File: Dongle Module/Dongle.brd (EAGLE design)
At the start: 45 x 28 mm, 31 parts, among them Q2 2.5A/30V, U1 RFM69HCW, U10 74AHC1G125, U8 ATSAMD21G-A, U9 3.3V, Y1 32.768kHz

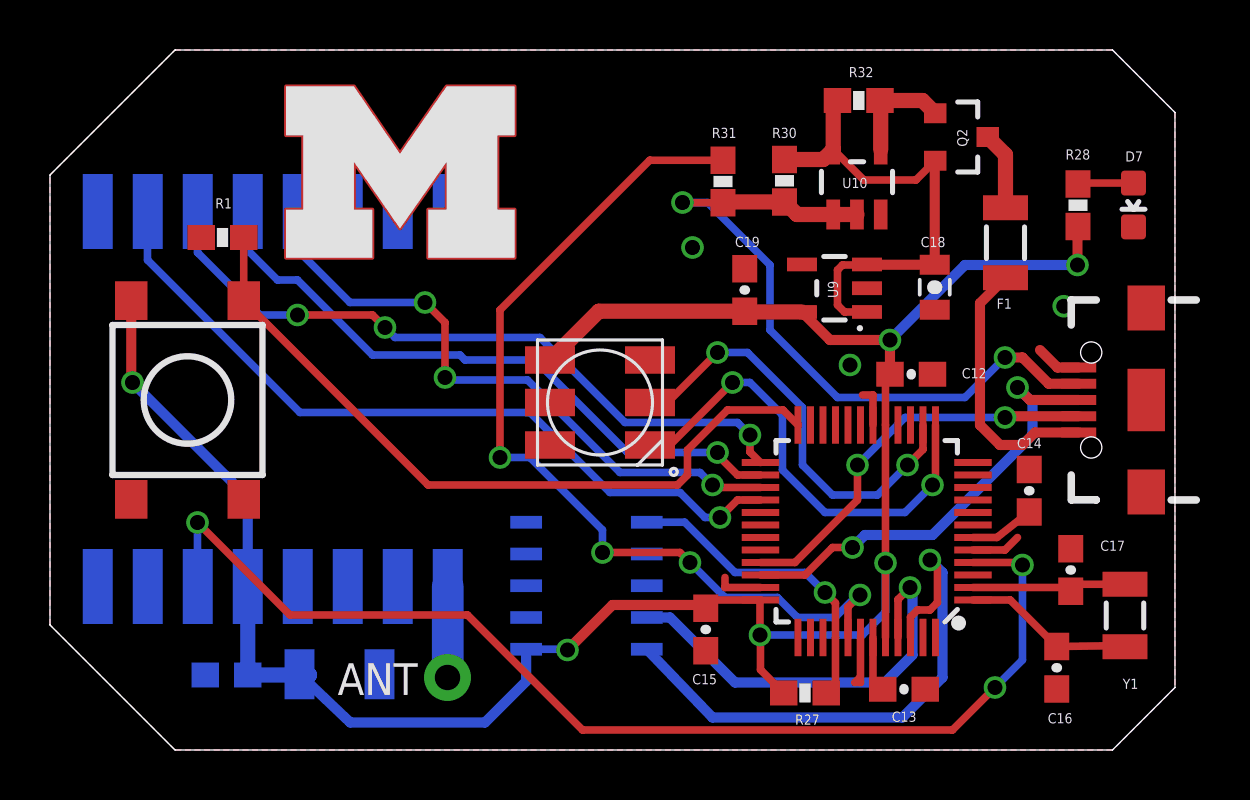
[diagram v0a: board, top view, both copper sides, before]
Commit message: ACTUALLY finalized all of the PCBs and created .zip's containing the gerber files of each
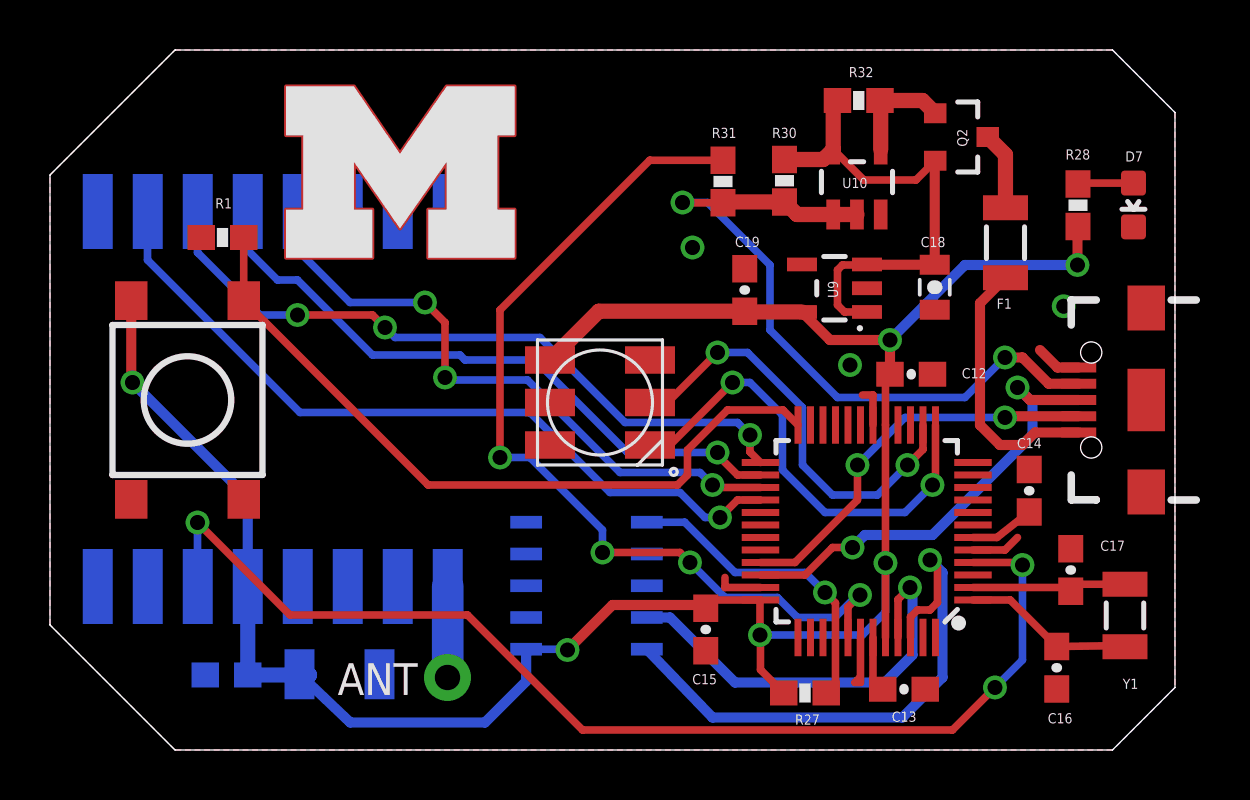
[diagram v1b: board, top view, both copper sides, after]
